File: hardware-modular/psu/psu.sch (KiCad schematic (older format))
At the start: 50 parts, among them J1 DC_OUT_1, J2 DC_OUT_2, J3 DC_OUT_3, J4 DC_OUT_4, J5 DC_IN, Q1 BD137, Q2 BD137, Q3 BD137, Q4 BD137, Q5 IRF9510, U1 L7805

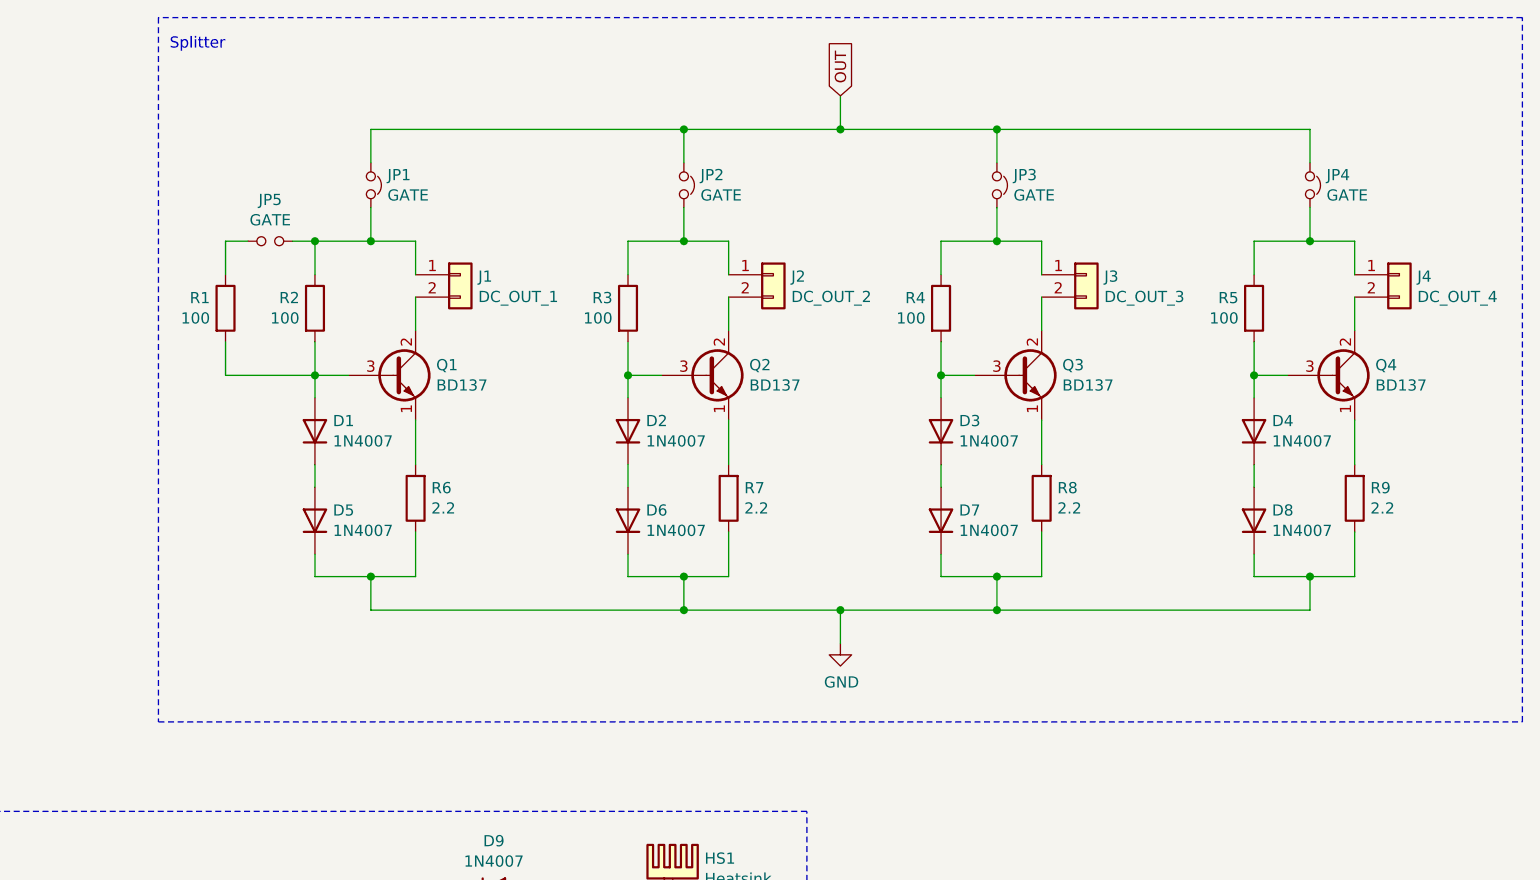
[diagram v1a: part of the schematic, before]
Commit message: PSU module revision.
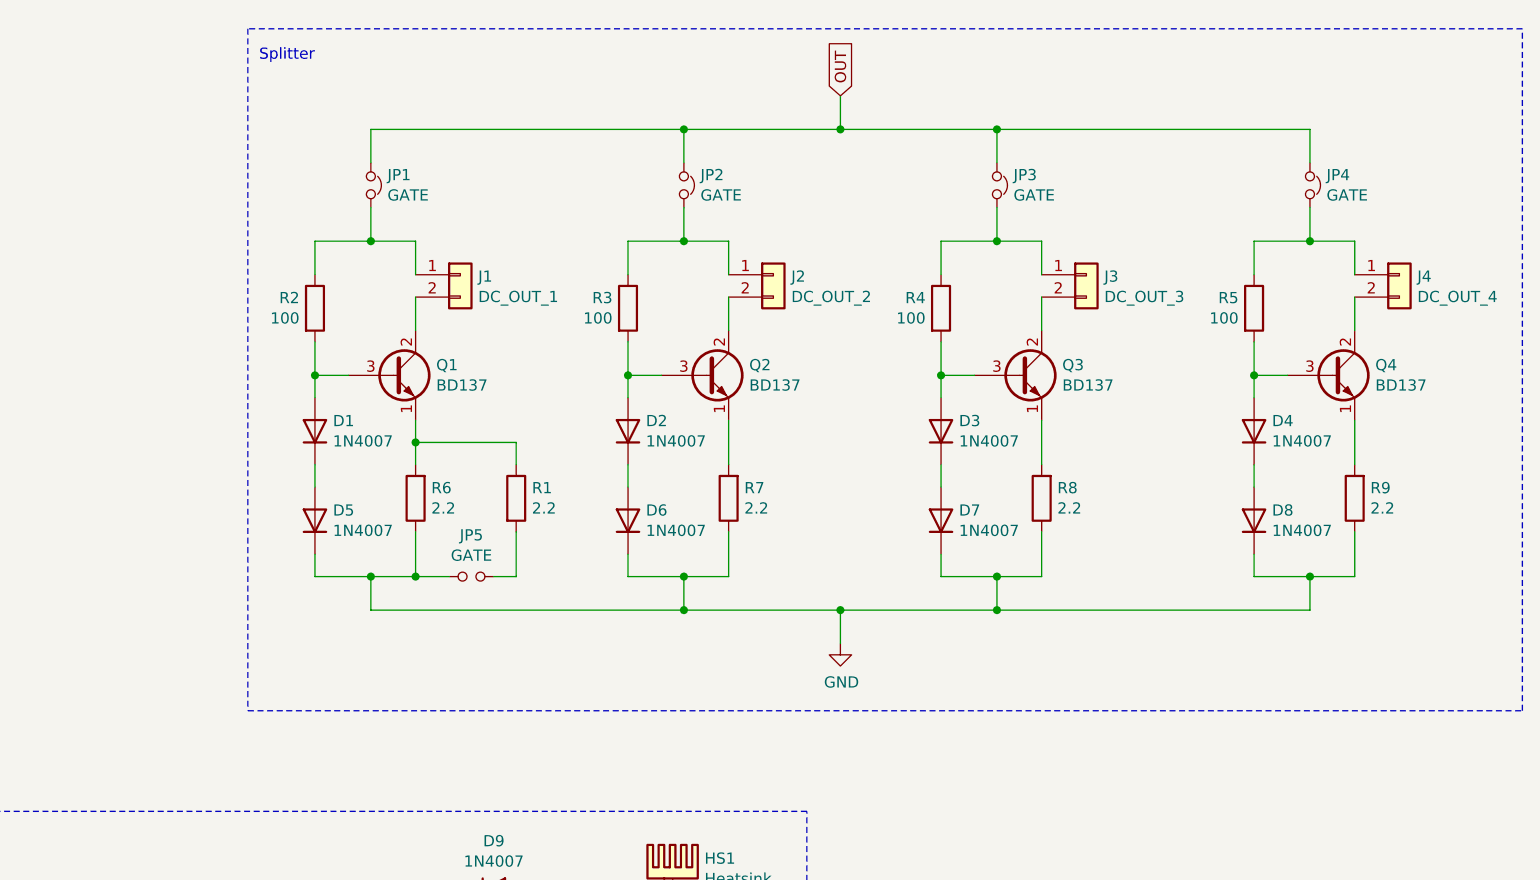
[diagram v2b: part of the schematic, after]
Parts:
- R1: value 100 -> 2.2; footprint Resistor_THT:R_Axial_DIN0207_L6.3mm_D2.5mm_P10.16mm_Horizontal -> Resistor_THT:R_Axial_DIN0309_L9.0mm_D3.2mm_P12.70mm_Horizontal
- R6: footprint Resistor_THT:R_Axial_DIN0207_L6.3mm_D2.5mm_P10.16mm_Horizontal -> Resistor_THT:R_Axial_DIN0309_L9.0mm_D3.2mm_P12.70mm_Horizontal
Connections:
- net GND: now also JP5.1
- net at J1.1 (Pin_1), JP1.2, R2.1: no longer JP5.2
- net at R1.1: now also Q1.1 (E), R6.2; no longer JP5.1
- net at D1.2 (A), Q1.3 (B), R2.2: no longer R1.2
- new net: JP5.2, R1.2
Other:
- moved on the sheet: JP5, R1
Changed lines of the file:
@@
 Text Notes 950  4750 0    50   ~ 0
 Regulator
-Text Notes 3700 1200 0    50   ~ 0
+Text Notes 4100 1250 0    50   ~ 0
 Splitter
 Wire Notes Line
-	9750 4200 9750 1050
+	9750 4150 9750 1100
 Wire Notes Line
-	9750 1050 3650 1050
+	9750 1100 4050 1100
 Wire Notes Line
-	3650 1050 3650 4200
+	4050 1100 4050 4150
 Wire Notes Line
-	3650 4200 9750 4200
+	4050 4150 9750 4150
 Wire Notes Line
 	6550 6800 6550 4600
@@
 F 3 "" H 1500 5900 50  0001 C CNN
 	1    1500 5900
-	1    0    0    -1
-$EndComp
-Connection ~ 4350 2050
-Wire Wire Line
-	4250 2050 4350 2050
-Wire Wire Line
-	3950 2050 4050 2050
-Wire Wire Line
-	3950 2200 3950 2050
-Wire Wire Line
-	3950 2650 3950 2500
-Wire Wire Line
-	4350 2650 3950 2650
-$Comp
-L Device:Jumper_NO_Small JP5
-U 1 1 60093A03
-P 4150 2050
-F 0 "JP5" H 4150 2235 50  0000 C CNN
-F 1 "GATE" H 4150 2144 50  0000 C CNN
-F 2 "Connector_PinHeader_2.54mm:PinHeader_1x02_P2.54mm_Vertical" H 4150 2050 50  0001 C CNN
-F 3 "~" H 4150 2050 50  0001 C CNN
-	1    4150 2050
-	1    0    0    -1
-$EndComp
-$Comp
-L Device:R R1
-U 1 1 60093359
-P 3950 2350
-F 0 "R1" H 3881 2396 50  0000 R CNN
-F 1 "100" H 3881 2305 50  0000 R CNN
-F 2 "Resistor_THT:R_Axial_DIN0207_L6.3mm_D2.5mm_P10.16mm_Horizontal" V 3880 2350 50  0001 C CNN
-F 3 "~" H 3950 2350 50  0001 C CNN
-	1    3950 2350
 	1    0    0    -1
 $EndComp
@@
 F 0 "R6" H 4730 3154 50  0000 R CNN
 F 1 "2.2" H 4730 3245 50  0000 R CNN
-F 2 "Resistor_THT:R_Axial_DIN0207_L6.3mm_D2.5mm_P10.16mm_Horizontal" V 4730 3200 50  0001 C CNN
+F 2 "Resistor_THT:R_Axial_DIN0309_L9.0mm_D3.2mm_P12.70mm_Horizontal" V 4730 3200 50  0001 C CNN
 F 3 "~" H 4800 3200 50  0001 C CNN
 	1    4800 3200
@@
 Wire Wire Line
 	4350 3550 4600 3550
-Wire Wire Line
-	4800 2850 4800 3050
 Wire Wire Line
 	4800 3350 4800 3550
@@
 	2200 6300 2700 6300
 Connection ~ 2200 6300
+Connection ~ 4800 3550
+Wire Wire Line
+	5250 3550 5250 3350
+Wire Wire Line
+	4800 3550 4950 3550
+Wire Wire Line
+	5250 2950 5250 3050
+$Comp
+L Device:R R1
+U 1 1 60093359
+P 5250 3200
+F 0 "R1" H 5320 3246 50  0000 L CNN
+F 1 "2.2" H 5320 3155 50  0000 L CNN
+F 2 "Resistor_THT:R_Axial_DIN0309_L9.0mm_D3.2mm_P12.70mm_Horizontal" V 5180 3200 50  0001 C CNN
+F 3 "~" H 5250 3200 50  0001 C CNN
+	1    5250 3200
+	1    0    0    -1
+$EndComp
+$Comp
+L Device:Jumper_NO_Small JP5
+U 1 1 60093A03
+P 5050 3550
+F 0 "JP5" H 5050 3735 50  0000 C CNN
+F 1 "GATE" H 5050 3644 50  0000 C CNN
+F 2 "Connector_PinHeader_2.54mm:PinHeader_1x02_P2.54mm_Vertical" H 5050 3550 50  0001 C CNN
+F 3 "~" H 5050 3550 50  0001 C CNN
+	1    5050 3550
+	1    0    0    -1
+$EndComp
+Wire Wire Line
+	5150 3550 5250 3550
+Wire Wire Line
+	4800 2950 5250 2950
+Wire Wire Line
+	4800 2850 4800 2950
+Connection ~ 4800 2950
+Wire Wire Line
+	4800 2950 4800 3050
 $EndSCHEMATC

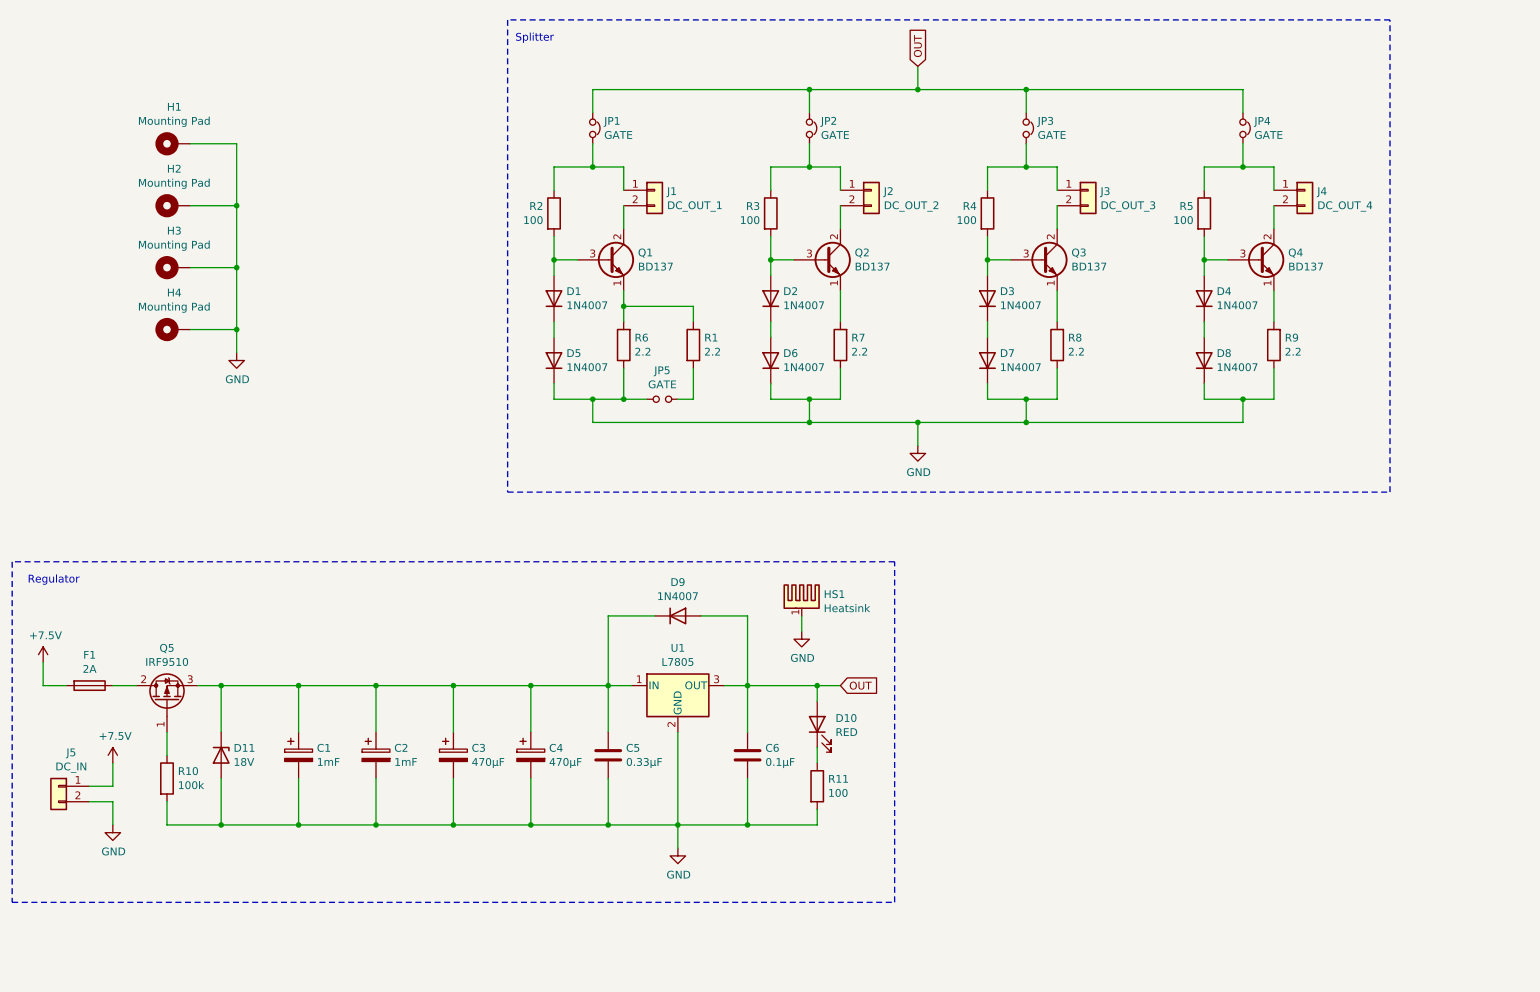
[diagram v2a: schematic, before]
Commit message: PSU module revision.
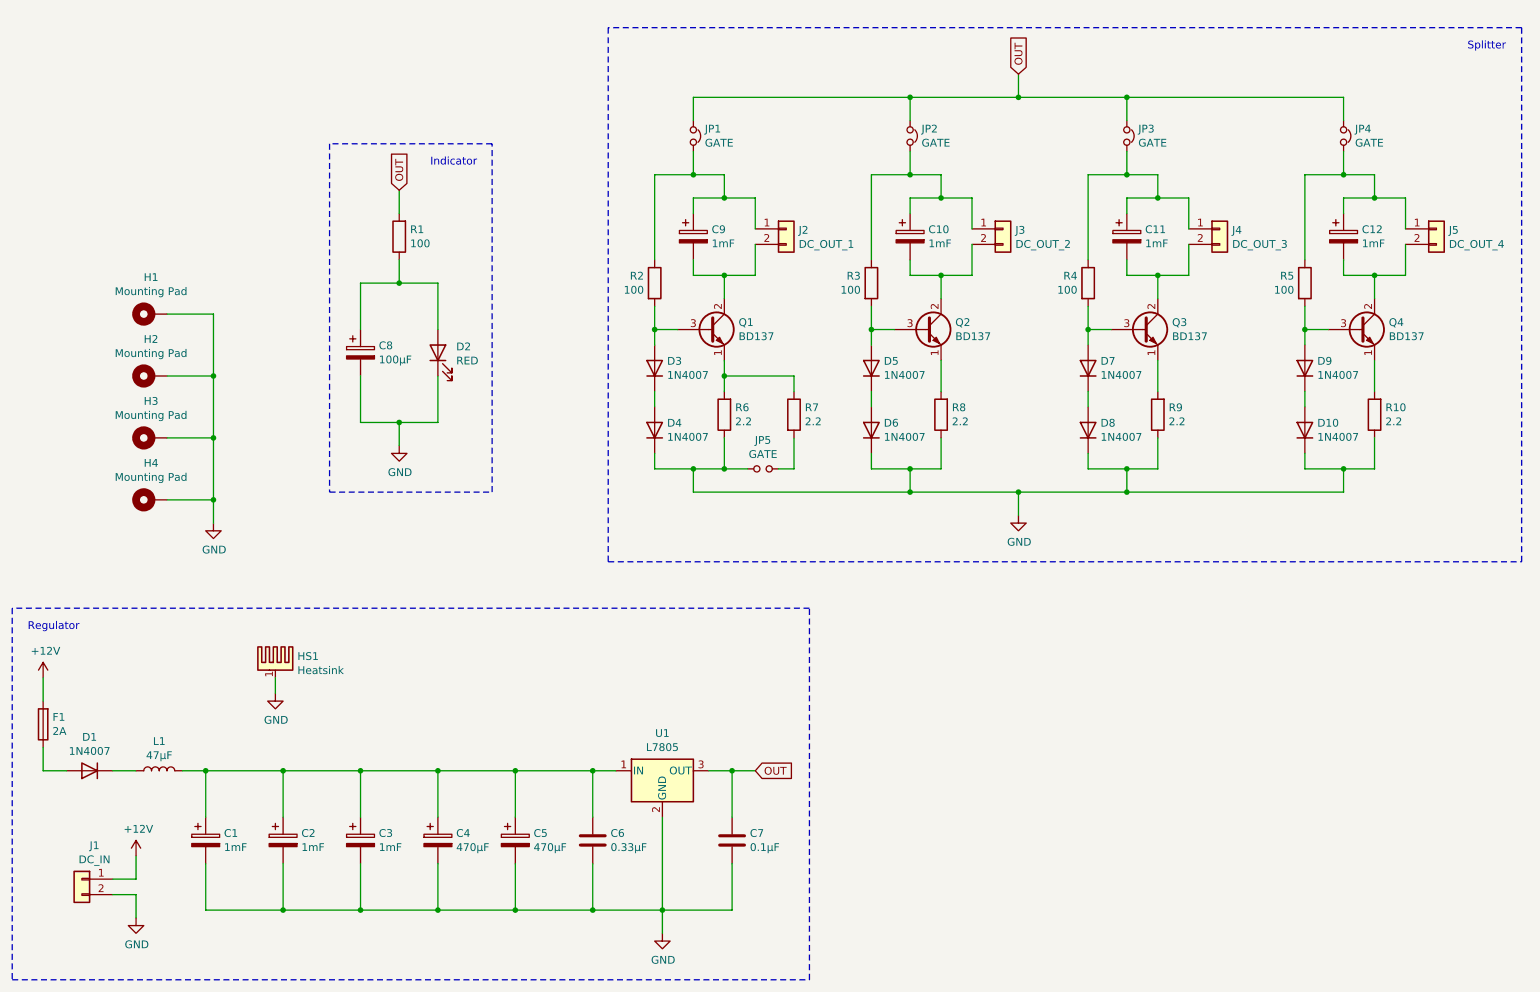
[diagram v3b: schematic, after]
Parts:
- removed D11: 18V, Diode_THT:D_DO-41_SOD81_P10.16mm_Horizontal, symbol Device:D_Zener
- removed D9: 1N4007, Diode_THT:D_DO-41_SOD81_P10.16mm_Horizontal, symbol Diode:1N4007
- removed Q5: IRF9510, Package_TO_SOT_THT:TO-220-3_Vertical, symbol Device:Q_PMOS_GDS
- removed R10: 100k, Resistor_THT:R_Axial_DIN0207_L6.3mm_D2.5mm_P10.16mm_Horizontal, symbol Device:R
- added C1: 1mF, Capacitor_THT:CP_Radial_D10.0mm_P5.00mm, symbol Device:CP
- added C10, C11, C12, C9: 1mF, Capacitor_THT:CP_Radial_D8.0mm_P3.50mm, symbol Device:CP
- added C8: 100µF, Capacitor_THT:CP_Radial_D5.0mm_P2.00mm, symbol Device:CP
- added D1: 1N4007, Diode_THT:D_DO-41_SOD81_P10.16mm_Horizontal, symbol Diode:1N4007
- added L1: 47µF, Inductor_THT:L_Toroid_Vertical_L16.0mm_W8.0mm_P7.62mm, symbol Device:L
- D10: renamed from D8; footprint Diode_THT:D_DO-41_SOD81_P10.16mm_Horizontal -> Diode_THT:D_DO-41_SOD81_P2.54mm_Vertical_AnodeUp
- D3: renamed from D1; footprint Diode_THT:D_DO-41_SOD81_P10.16mm_Horizontal -> Diode_THT:D_DO-41_SOD81_P2.54mm_Vertical_AnodeUp
- D4: renamed from D5; footprint Diode_THT:D_DO-41_SOD81_P10.16mm_Horizontal -> Diode_THT:D_DO-41_SOD81_P2.54mm_Vertical_AnodeUp
- D5: renamed from D2; footprint Diode_THT:D_DO-41_SOD81_P10.16mm_Horizontal -> Diode_THT:D_DO-41_SOD81_P2.54mm_Vertical_AnodeUp
- D6: footprint Diode_THT:D_DO-41_SOD81_P10.16mm_Horizontal -> Diode_THT:D_DO-41_SOD81_P2.54mm_Vertical_AnodeUp
- D7: renamed from D3; footprint Diode_THT:D_DO-41_SOD81_P10.16mm_Horizontal -> Diode_THT:D_DO-41_SOD81_P2.54mm_Vertical_AnodeUp
- D8: renamed from D7; footprint Diode_THT:D_DO-41_SOD81_P10.16mm_Horizontal -> Diode_THT:D_DO-41_SOD81_P2.54mm_Vertical_AnodeUp
- D9: renamed from D4; footprint Diode_THT:D_DO-41_SOD81_P10.16mm_Horizontal -> Diode_THT:D_DO-41_SOD81_P2.54mm_Vertical_AnodeUp
- renumbered C1 to C2, C2 to C3, C3 to C4, C4 to C5, C5 to C6, C6 to C7, D10 to D2, J5 to J1, J1 to J2, J2 to J3, J3 to J4, J4 to J5, R11 to R1, R9 to R10, R1 to R7, R7 to R8, R8 to R9
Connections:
- net GND: now also D2.1 (K), C1.2, C8.2; no longer R1.2
- net OUT: now also R1.2; no longer D2.2 (A)
- net at C2.1, C3.1, C4.1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: now also C1.1, L1.2
- net at J2.1 (Pin_1), JP1.2, R2.1: now also C9.1
- net at J2.2 (Pin_2), Q1.2 (C): now also C9.2
- net at J3.1 (Pin_1), JP2.2, R3.1: now also C10.1
- net at J3.2 (Pin_2), Q2.2 (C): now also C10.2
- net at J5.1 (Pin_1), JP4.2, R5.1: now also C12.1
- net at J5.2 (Pin_2), Q4.2 (C): now also C12.2
- net at J4.1 (Pin_1), JP3.2, R4.1: now also C11.1
- net at J4.2 (Pin_2), Q3.2 (C): now also C11.2
- net at F1.1: now also D1.2 (A)
- net at R1.1: now also D2.2 (A), C8.1; no longer D2.1 (K)
- net +7.5V renamed +12V
- new net: D1.1 (K), L1.1
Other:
- note added: "Indicator"
- moved on the sheet: C2, C3, C4, C5, C6, C7, D10, D2, D3, D4, D5, D6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
